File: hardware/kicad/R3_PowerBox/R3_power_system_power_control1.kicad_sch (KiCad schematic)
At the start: 7 parts, among them Q4 DMP3007LSS-13 SYSTEM LOAD SWI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, SW1 C&K RS282G05A3 / POWER ON

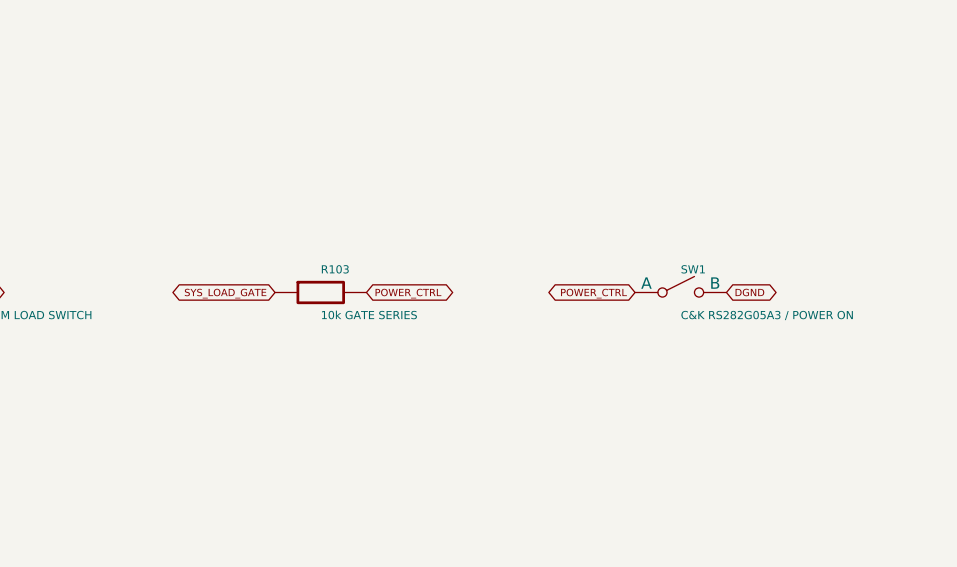
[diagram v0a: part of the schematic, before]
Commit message: Rev.A review fixes: local charger power-stage reroute checkpoint
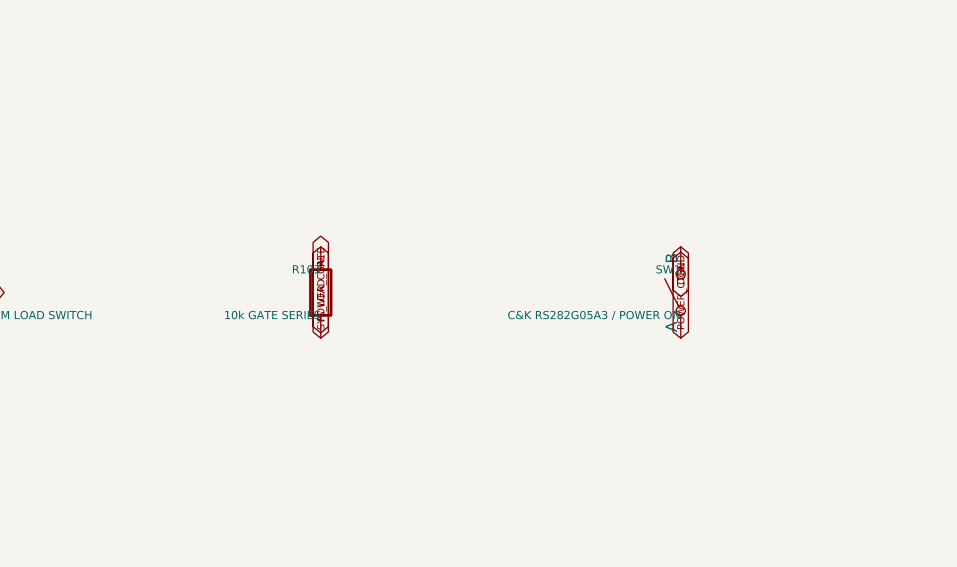
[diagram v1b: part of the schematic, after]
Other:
- moved on the sheet: R103, SW1
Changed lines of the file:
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@@
 	(global_label "SYS_LOAD_GATE"
 		(shape bidirectional)
-		(at 179.92 105 180)
+		(at 185 110.08 90)
+		(effects
+			(font
+				(size 0.8 0.8)
+			)
+			(justify left)
+		)
+	)
+	(global_label "POWER_CTRL"
+		(shape bidirectional)
+		(at 185 99.92 270)
 		(effects
 			(font
@@
 	(global_label "POWER_CTRL"
 		(shape bidirectional)
-		(at 190.08 105 0)
+		(at 225 110.08 90)
 		(effects
 			(font
@@
 		)
 	)
-	(global_label "POWER_CTRL"
-		(shape bidirectional)
-		(at 219.92 105 180)
+	(global_label "DGND"
+		(shape bidirectional)
+		(at 225 99.92 270)
 		(effects
 			(font
@@
 			)
 			(justify right)
-		)
-	)
-	(global_label "DGND"
-		(shape bidirectional)
-		(at 230.08 105 0)
-		(effects
-			(font
-				(size 0.8 0.8)
-			)
-			(justify left)
 		)
 	)
@@
     (instances
       (project "SKiDL-Generated"
-        (path "/7d40ec76-f97b-4a90-b5ea-ddf1628062b5/a9caf0ad-ee07-5321-84f1-7681c239e759"
+        (path "/2b0a7443-ac4c-4207-8273-267cee2a0847/a9caf0ad-ee07-5321-84f1-7681c239e759"
           (reference "Q4")
           (unit 1)))))
@@
     (instances
       (project "SKiDL-Generated"
-        (path "/7d40ec76-f97b-4a90-b5ea-ddf1628062b5/a9caf0ad-ee07-5321-84f1-7681c239e759"
+        (path "/2b0a7443-ac4c-4207-8273-267cee2a0847/a9caf0ad-ee07-5321-84f1-7681c239e759"
           (reference "R102")
           (unit 1)))))
@@
     (instances
       (project "SKiDL-Generated"
-        (path "/7d40ec76-f97b-4a90-b5ea-ddf1628062b5/a9caf0ad-ee07-5321-84f1-7681c239e759"
+        (path "/2b0a7443-ac4c-4207-8273-267cee2a0847/a9caf0ad-ee07-5321-84f1-7681c239e759"
           (reference "C107")
           (unit 1)))))
   (symbol
     (lib_id "R3_POWER_GEN:R")
-    (at 185 105 0)
+    (at 185 105 90)
     (unit 1)
     (exclude_from_sim no)
@@
     (fields_autoplaced yes)
     (property "Reference" "R103"
-      (at 185 102.46 0)
+      (at 185 102.46 90)
       (effects
         (font
@@
         (justify left)))
     (property "Value" "10k GATE SERIES"
-      (at 185 107.54 0)
+      (at 185 107.54 90)
       (effects
         (font
@@
         (justify left)))
     (property "Footprint" "Resistor_SMD:R_0603_1608Metric"
-      (at 185 105 0)
-      (effects
-        (font
-          (size 0.9 0.9))
-        (hide yes)))
-    (property "Datasheet" "~"
-      (at 185 105 0)
-      (effects
-        (font
-          (size 0.9 0.9))
-        (hide yes)))
-    (property "Description" ""
-      (at 185 105 0)
-      (effects
-        (font
-          (size 0.9 0.9))
-        (hide yes)))
-    (pin "1"
-)
-    (pin "2"
-)
-    (instances
-      (project "SKiDL-Generated"
-        (path "/7d40ec76-f97b-4a90-b5ea-ddf1628062b5/a9caf0ad-ee07-5321-84f1-7681c239e759"
+      (at 185 105 90)
+      (effects
+        (font
+          (size 0.9 0.9))
+        (hide yes)))
+    (property "Datasheet" "~"
+      (at 185 105 90)
+      (effects
+        (font
+          (size 0.9 0.9))
+        (hide yes)))
+    (property "Description" ""
+      (at 185 105 90)
+      (effects
+        (font
+          (size 0.9 0.9))
+        (hide yes)))
+    (pin "1"
+)
+    (pin "2"
+)
+    (instances
+      (project "SKiDL-Generated"
+        (path "/2b0a7443-ac4c-4207-8273-267cee2a0847/a9caf0ad-ee07-5321-84f1-7681c239e759"
           (reference "R103")
           (unit 1)))))
   (symbol
     (lib_id "Switch:SW_SPST")
-    (at 225 105 0)
+    (at 225 105 90)
     (unit 1)
     (exclude_from_sim no)
@@
     (fields_autoplaced yes)
     (property "Reference" "SW1"
-      (at 225 102.46 0)
+      (at 225 102.46 90)
       (effects
         (font
@@
         (justify left)))
     (property "Value" "C&K RS282G05A3 / POWER ON"
-      (at 225 107.54 0)
+      (at 225 107.54 90)
       (effects
         (font
@@
         (justify left)))
     (property "Footprint" "Button_Switch_SMD:SW_SPST_CK_RS282G05A3"
-      (at 225 105 0)
-      (effects
-        (font
-          (size 0.9 0.9))
-        (hide yes)))
-    (property "Datasheet" "~"
-      (at 225 105 0)
+      (at 225 105 90)
+      (effects
+        (font
+          (size 0.9 0.9))
+        (hide yes)))
+    (property "Datasheet" "~"
+      (at 225 105 90)
       (effects
         (font
@@
         (hide yes)))
     (property "Description" "Single Pole Single Throw (SPST) switch"
-      (at 225 105 0)
-      (effects
-        (font
-          (size 0.9 0.9))
-        (hide yes)))
-    (pin "1"
-)
-    (pin "2"
-)
-    (instances
-      (project "SKiDL-Generated"
-        (path "/7d40ec76-f97b-4a90-b5ea-ddf1628062b5/a9caf0ad-ee07-5321-84f1-7681c239e759"
+      (at 225 105 90)
+      (effects
+        (font
+          (size 0.9 0.9))
+        (hide yes)))
+    (pin "1"
+)
+    (pin "2"
+)
+    (instances
+      (project "SKiDL-Generated"
+        (path "/2b0a7443-ac4c-4207-8273-267cee2a0847/a9caf0ad-ee07-5321-84f1-7681c239e759"
           (reference "SW1")
           (unit 1)))))
@@
     (instances
       (project "SKiDL-Generated"
-        (path "/7d40ec76-f97b-4a90-b5ea-ddf1628062b5/a9caf0ad-ee07-5321-84f1-7681c239e759"
+        (path "/2b0a7443-ac4c-4207-8273-267cee2a0847/a9caf0ad-ee07-5321-84f1-7681c239e759"
           (reference "C108")
           (unit 1)))))
@@
     (instances
       (project "SKiDL-Generated"
-        (path "/7d40ec76-f97b-4a90-b5ea-ddf1628062b5/a9caf0ad-ee07-5321-84f1-7681c239e759"
+        (path "/2b0a7443-ac4c-4207-8273-267cee2a0847/a9caf0ad-ee07-5321-84f1-7681c239e759"
           (reference "TP40")
           (unit 1)))))
